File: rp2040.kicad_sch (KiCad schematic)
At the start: 8 parts, among them U1 RP2040, Y1 12 MHz

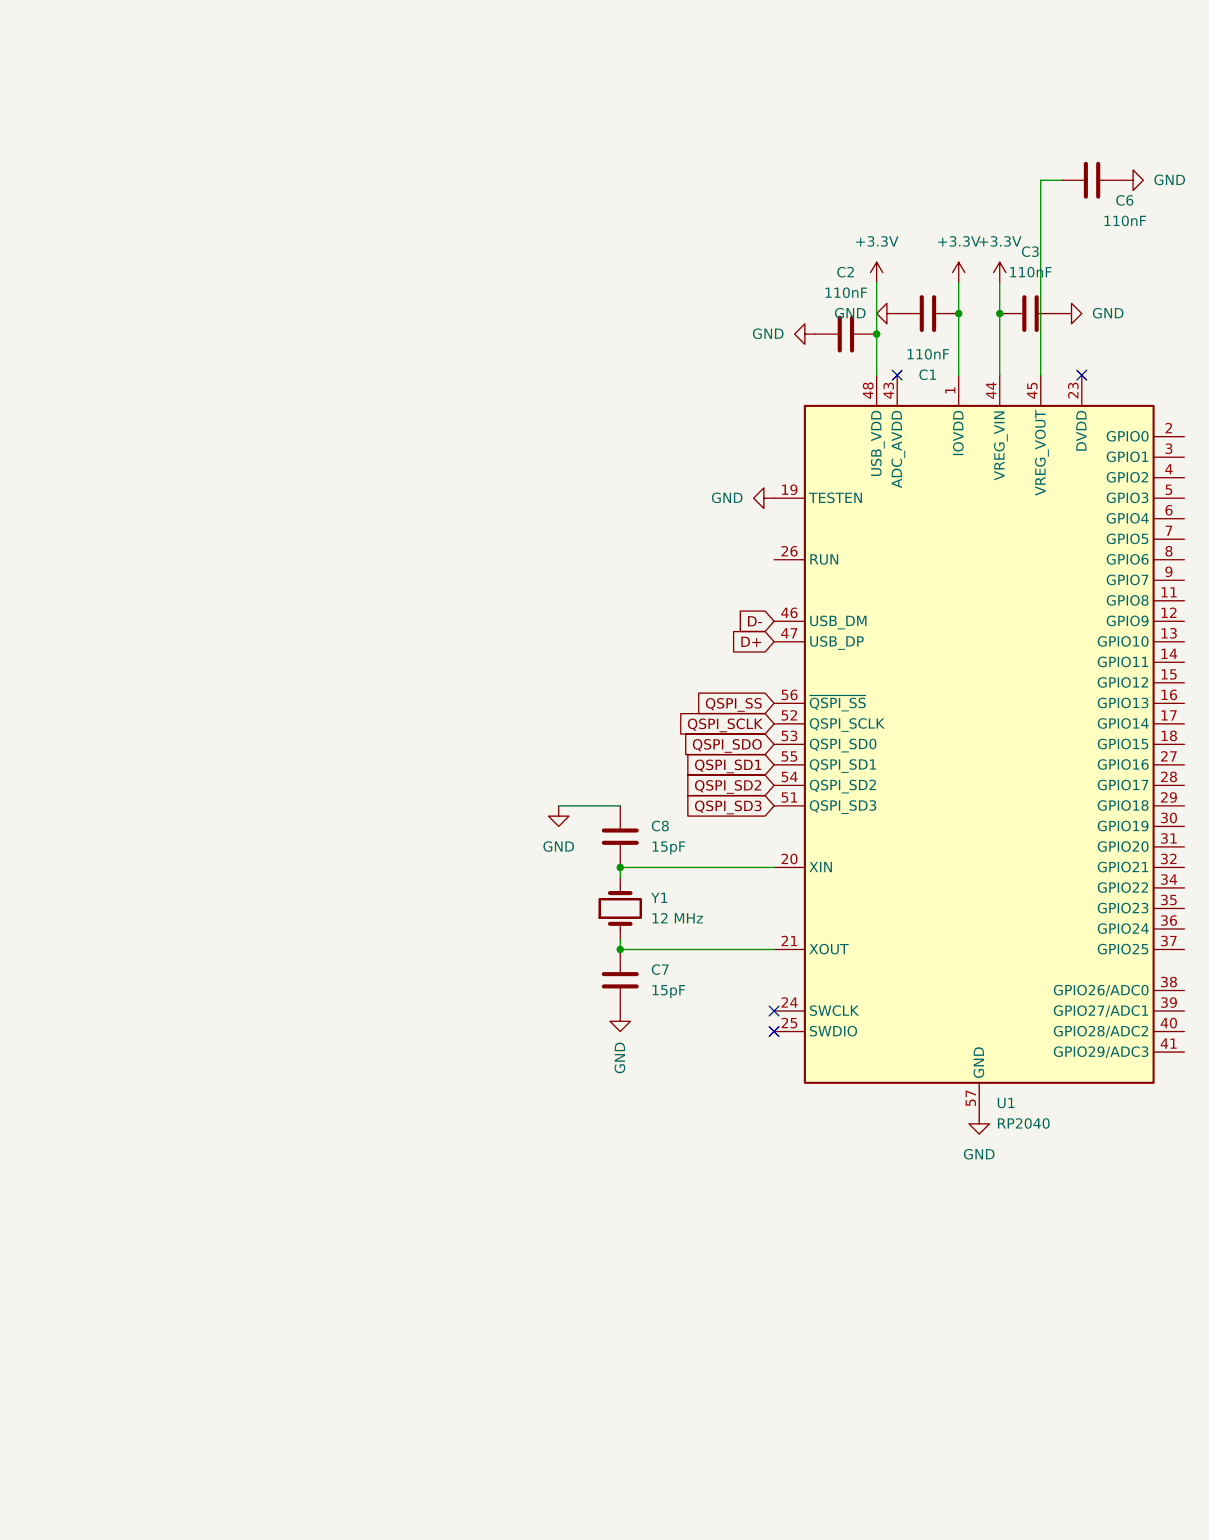
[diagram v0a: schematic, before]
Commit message: Savepoint!
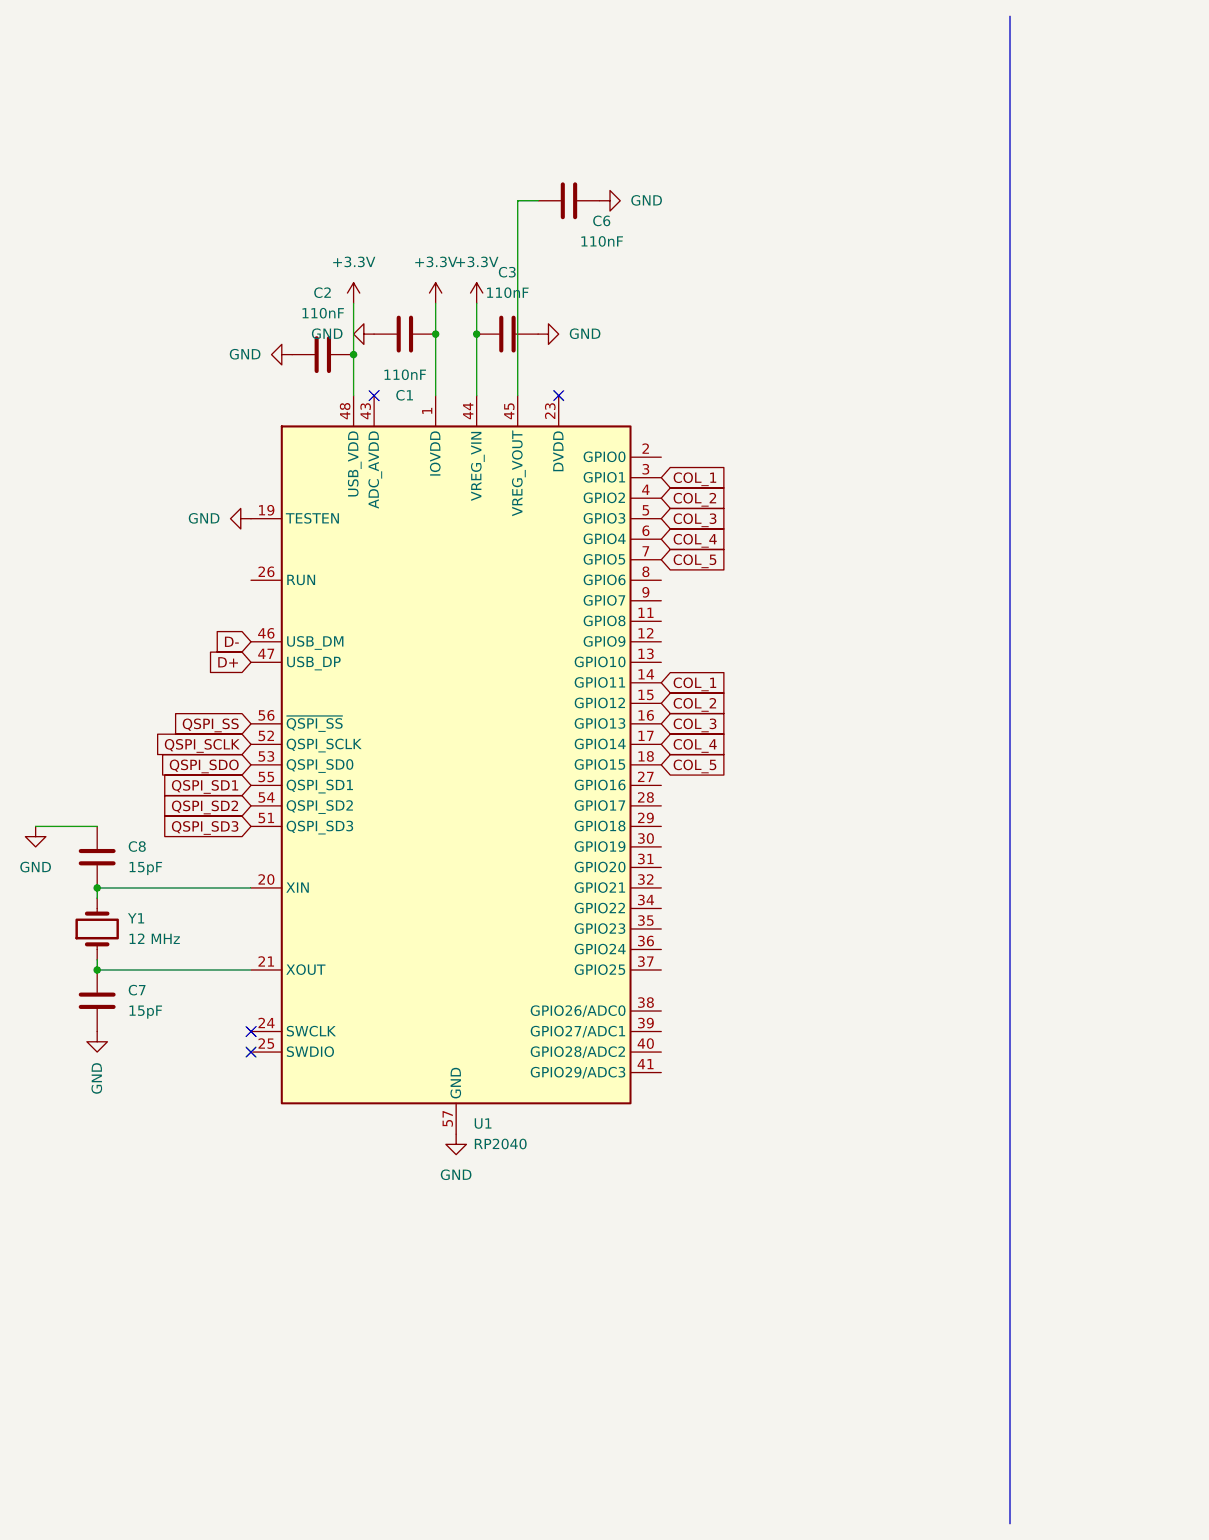
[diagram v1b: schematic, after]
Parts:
- C1, C2, C3, C6: footprint (none) -> Capacitor_Tantalum_SMD:CP_EIA-1608-08_AVX-J_HandSolder
- C7, C8: footprint (none) -> Capacitor_SMD:C_0402_1005Metric_Pad0.74x0.62mm_HandSolder
- Y1: footprint (none) -> Crystal:Crystal_SMD_3225-4Pin_3.2x2.5mm_HandSoldering
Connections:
- net COL_1: now reaches U1.14 (GPIO11)
- net COL_1: now also U1.3 (GPIO1)
- net COL_2: now reaches U1.15 (GPIO12)
- net COL_2: now also U1.4 (GPIO2)
- net COL_3: now reaches U1.16 (GPIO13)
- net COL_3: now also U1.5 (GPIO3)
- net COL_4: now reaches U1.17 (GPIO14)
- net COL_4: now also U1.6 (GPIO4)
- net COL_5: now reaches U1.18 (GPIO15)
- net COL_5: now also U1.7 (GPIO5)
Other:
- moved on the sheet: C1, C2, C3, C6, C7, C8, U1, Y1

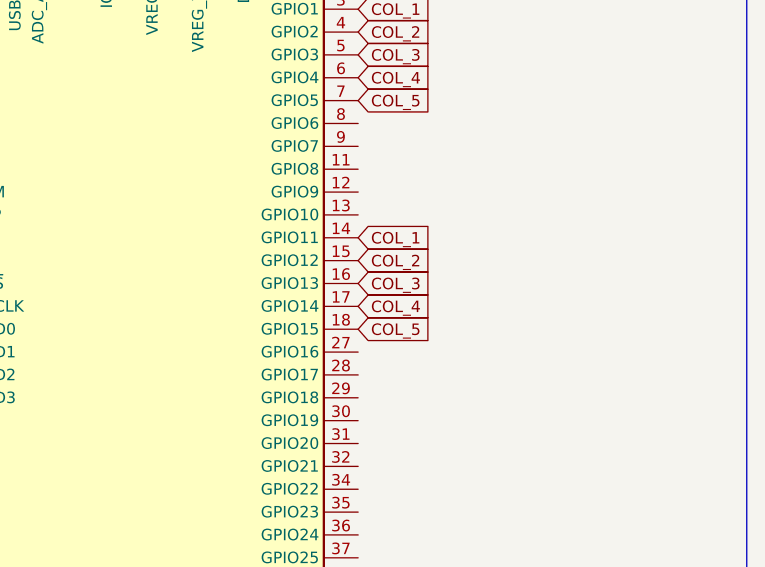
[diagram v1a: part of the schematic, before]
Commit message: Savepoint!
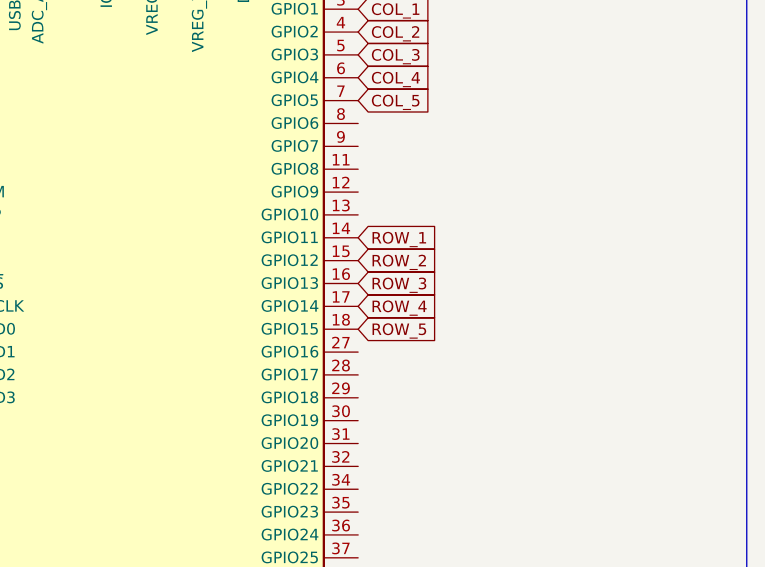
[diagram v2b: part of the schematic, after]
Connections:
- net COL_1: no longer U1.14 (GPIO11)
- net COL_2: no longer U1.15 (GPIO12)
- net COL_3: no longer U1.16 (GPIO13)
- net COL_4: no longer U1.17 (GPIO14)
- net COL_5: no longer U1.18 (GPIO15)
- new net ROW_1: U1.14 (GPIO11)
- new net ROW_2: U1.15 (GPIO12)
- new net ROW_3: U1.16 (GPIO13)
- new net ROW_4: U1.17 (GPIO14)
- new net ROW_5: U1.18 (GPIO15)
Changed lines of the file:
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@@
+		)
+	)
+	(global_label "ROW_3"
+		(shape input)
+		(at 105.41 99.06 0)
+		(fields_autoplaced yes)
+		(effects
+			(font
+				(size 1.27 1.27)
+			)
+			(justify left)
+		)
+		(property "Intersheetrefs" "${INTERSHEET_REFS}"
+			(at 114.6242 99.06 0)
+			(hide yes)
+			(show_name no)
+			(do_not_autoplace no)
+			(effects
+				(font
+					(size 1.27 1.27)
+				)
+				(justify left)
+			)
+		)
+	)
+	(global_label "QSPI_SD3"
+		(shape input)
+		(at 54.61 111.76 180)
+		(fields_autoplaced yes)
+		(effects
+			(font
+				(size 1.27 1.27)
+			)
+			(justify right)
+		)
+		(property "Intersheetrefs" "${INTERSHEET_REFS}"
+			(at 42.5534 111.76 0)
+			(hide yes)
+			(show_name no)
+			(do_not_autoplace no)
+			(effects
+				(font
+					(size 1.27 1.27)
+				)
+				(justify right)
+			)
+		)
+	)
+	(global_label "QSPI_SD2"
+		(shape input)
+		(at 54.61 109.22 180)
+		(fields_autoplaced yes)
+		(effects
+			(font
+				(size 1.27 1.27)
+			)
+			(justify right)
+		)
+		(property "Intersheetrefs" "${INTERSHEET_REFS}"
+			(at 42.5534 109.22 0)
+			(hide yes)
+			(show_name no)
+			(do_not_autoplace no)
+			(effects
+				(font
+					(size 1.27 1.27)
+				)
+				(justify right)
+			)
+		)
+	)
+	(global_label "COL_1"
+		(shape input)
+		(at 105.41 68.58 0)
+		(fields_autoplaced yes)
+		(effects
+			(font
+				(size 1.27 1.27)
+			)
+			(justify left)
+		)
+		(property "Intersheetrefs" "${INTERSHEET_REFS}"
+			(at 114.2009 68.58 0)
+			(hide yes)
+			(show_name no)
+			(do_not_autoplace no)
+			(effects
+				(font
+					(size 1.27 1.27)
+				)
+				(justify left)
+			)
+		)
+	)
+	(global_label "COL_2"
+		(shape input)
+		(at 105.41 71.12 0)
+		(fields_autoplaced yes)
+		(effects
+			(font
+				(size 1.27 1.27)
+			)
+			(justify left)
+		)
+		(property "Intersheetrefs" "${INTERSHEET_REFS}"
+			(at 114.2009 71.12 0)
+			(hide yes)
+			(show_name no)
+			(do_not_autoplace no)
+			(effects
+				(font
+					(size 1.27 1.27)
+				)
+				(justify left)
+			)
+		)
+	)
+	(global_label "ROW_5"
+		(shape input)
+		(at 105.41 104.14 0)
+		(fields_autoplaced yes)
+		(effects
+			(font
+				(size 1.27 1.27)
+			)
+			(justify left)
+		)
+		(property "Intersheetrefs" "${INTERSHEET_REFS}"
+			(at 114.6242 104.14 0)
+			(hide yes)
+			(show_name no)
+			(do_not_autoplace no)
+			(effects
+				(font
+					(size 1.27 1.27)
+				)
+				(justify left)
+			)
+		)
+	)
+	(global_label "COL_5"
+		(shape input)
+		(at 105.41 78.74 0)
+		(fields_autoplaced yes)
+		(effects
+			(font
+				(size 1.27 1.27)
+			)
+			(justify left)
+		)
+		(property "Intersheetrefs" "${INTERSHEET_REFS}"
+			(at 114.2009 78.74 0)
+			(hide yes)
+			(show_name no)
+			(do_not_autoplace no)
+			(effects
+				(font
+					(size 1.27 1.27)
+				)
+				(justify left)
+			)
+		)
+	)
+	(global_label "QSPI_SS"
+		(shape input)
+		(at 54.61 99.06 180)
+		(fields_autoplaced yes)
+		(effects
+			(font
+				(size 1.27 1.27)
+			)
+			(justify right)
+		)
+		(property "Intersheetrefs" "${INTERSHEET_REFS}"
+			(at 43.8234 99.06 0)
+			(hide yes)
+			(show_name no)
+			(do_not_autoplace no)
+			(effects
+				(font
+					(size 1.27 1.27)
+				)
+				(justify right)
+			)
 		)
 	)
 	(global_label "COL_3"
 		(shape input)
-		(at 105.41 99.06 0)
-		(fields_autoplaced yes)
-		(effects
-			(font
-				(size 1.27 1.27)
-			)
-			(justify left)
-		)
-		(property "Intersheetrefs" "${INTERSHEET_REFS}"
-			(at 114.2009 99.06 0)
-			(hide yes)
-			(show_name no)
-			(do_not_autoplace no)
-			(effects
-				(font
-					(size 1.27 1.27)
-				)
-				(justify left)
-			)
-		)
-	)
-	(global_label "QSPI_SD3"
-		(shape input)
-		(at 54.61 111.76 180)
-		(fields_autoplaced yes)
-		(effects
-			(font
-				(size 1.27 1.27)
-			)
-			(justify right)
-		)
-		(property "Intersheetrefs" "${INTERSHEET_REFS}"
-			(at 42.5534 111.76 0)
-			(hide yes)
-			(show_name no)
-			(do_not_autoplace no)
-			(effects
-				(font
-					(size 1.27 1.27)
-				)
-				(justify right)
-			)
-		)
-	)
-	(global_label "QSPI_SD2"
-		(shape input)
-		(at 54.61 109.22 180)
-		(fields_autoplaced yes)
-		(effects
-			(font
-				(size 1.27 1.27)
-			)
-			(justify right)
-		)
-		(property "Intersheetrefs" "${INTERSHEET_REFS}"
-			(at 42.5534 109.22 0)
-			(hide yes)
-			(show_name no)
-			(do_not_autoplace no)
-			(effects
-				(font
-					(size 1.27 1.27)
-				)
-				(justify right)
-			)
-		)
-	)
-	(global_label "COL_1"
-		(shape input)
-		(at 105.41 68.58 0)
-		(fields_autoplaced yes)
-		(effects
-			(font
-				(size 1.27 1.27)
-			)
-			(justify left)
-		)
-		(property "Intersheetrefs" "${INTERSHEET_REFS}"
-			(at 114.2009 68.58 0)
-			(hide yes)
-			(show_name no)
-			(do_not_autoplace no)
-			(effects
-				(font
-					(size 1.27 1.27)
-				)
-				(justify left)
-			)
-		)
-	)
-	(global_label "COL_2"
-		(shape input)
-		(at 105.41 71.12 0)
-		(fields_autoplaced yes)
-		(effects
-			(font
-				(size 1.27 1.27)
-			)
-			(justify left)
-		)
-		(property "Intersheetrefs" "${INTERSHEET_REFS}"
-			(at 114.2009 71.12 0)
-			(hide yes)
-			(show_name no)
-			(do_not_autoplace no)
-			(effects
-				(font
-					(size 1.27 1.27)
-				)
-				(justify left)
-			)
-		)
-	)
-	(global_label "COL_5"
-		(shape input)
-		(at 105.41 104.14 0)
-		(fields_autoplaced yes)
-		(effects
-			(font
-				(size 1.27 1.27)
-			)
-			(justify left)
-		)
-		(property "Intersheetrefs" "${INTERSHEET_REFS}"
-			(at 114.2009 104.14 0)
-			(hide yes)
-			(show_name no)
-			(do_not_autoplace no)
-			(effects
-				(font
-					(size 1.27 1.27)
-				)
-				(justify left)
-			)
-		)
-	)
-	(global_label "COL_5"
-		(shape input)
-		(at 105.41 78.74 0)
-		(fields_autoplaced yes)
-		(effects
-			(font
-				(size 1.27 1.27)
-			)
-			(justify left)
-		)
-		(property "Intersheetrefs" "${INTERSHEET_REFS}"
-			(at 114.2009 78.74 0)
-			(hide yes)
-			(show_name no)
-			(do_not_autoplace no)
-			(effects
-				(font
-					(size 1.27 1.27)
-				)
-				(justify left)
-			)
-		)
-	)
-	(global_label "QSPI_SS"
-		(shape input)
-		(at 54.61 99.06 180)
-		(fields_autoplaced yes)
-		(effects
-			(font
-				(size 1.27 1.27)
-			)
-			(justify right)
-		)
-		(property "Intersheetrefs" "${INTERSHEET_REFS}"
-			(at 43.8234 99.06 0)
-			(hide yes)
-			(show_name no)
-			(do_not_autoplace no)
-			(effects
-				(font
-					(size 1.27 1.27)
-				)
-				(justify right)
-			)
-		)
-	)
-	(global_label "COL_3"
-		(shape input)
 		(at 105.41 73.66 0)
 		(fields_autoplaced yes)
@@
 		)
 	)
-	(global_label "COL_4"
+	(global_label "ROW_4"
 		(shape input)
 		(at 105.41 101.6 0)
@@
 		)
 		(property "Intersheetrefs" "${INTERSHEET_REFS}"
-			(at 114.2009 101.6 0)
-			(hide yes)
-			(show_name no)
-			(do_not_autoplace no)
-			(effects
-				(font
-					(size 1.27 1.27)
-				)
-				(justify left)
-			)
-		)
-	)
-	(global_label "COL_2"
+			(at 114.6242 101.6 0)
+			(hide yes)
+			(show_name no)
+			(do_not_autoplace no)
+			(effects
+				(font
+					(size 1.27 1.27)
+				)
+				(justify left)
+			)
+		)
+	)
+	(global_label "ROW_2"
 		(shape input)
 		(at 105.41 96.52 0)
@@
 		)
 		(property "Intersheetrefs" "${INTERSHEET_REFS}"
-			(at 114.2009 96.52 0)
+			(at 114.6242 96.52 0)
 			(hide yes)
 			(show_name no)
@@
 		)
 	)
-	(global_label "COL_1"
+	(global_label "ROW_1"
 		(shape input)
 		(at 105.41 93.98 0)
@@
 		)
 		(property "Intersheetrefs" "${INTERSHEET_REFS}"
-			(at 114.2009 93.98 0)
-			(hide yes)
-			(show_name no)
+			(at 114.6242 93.98 0)
+			(hide yes)
+			(show_name no)

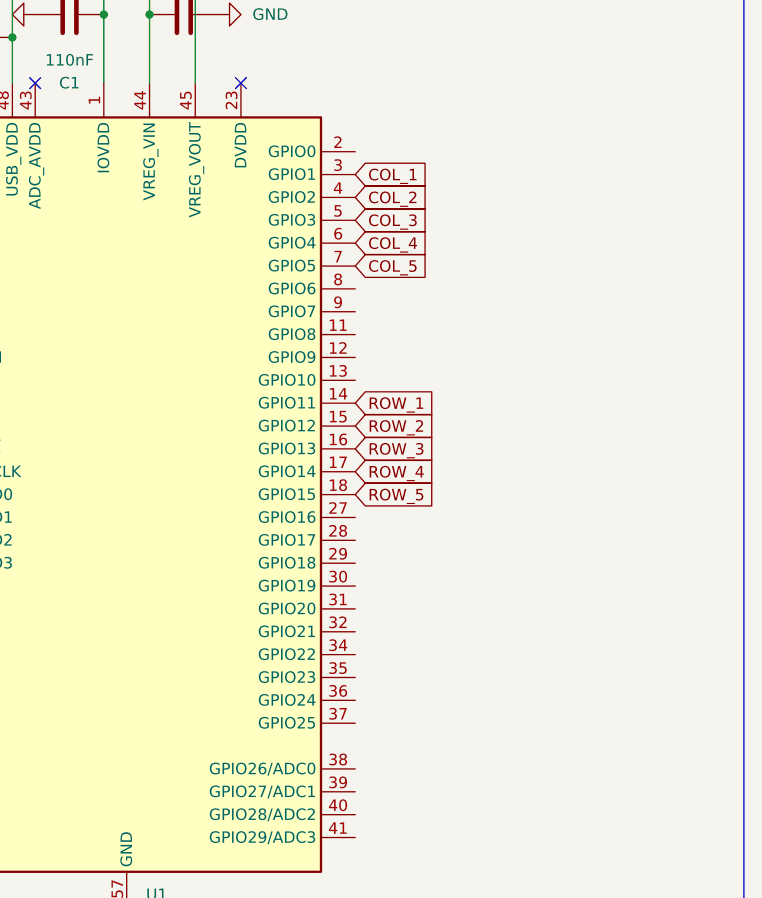
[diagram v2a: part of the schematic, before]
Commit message: Savepoint!
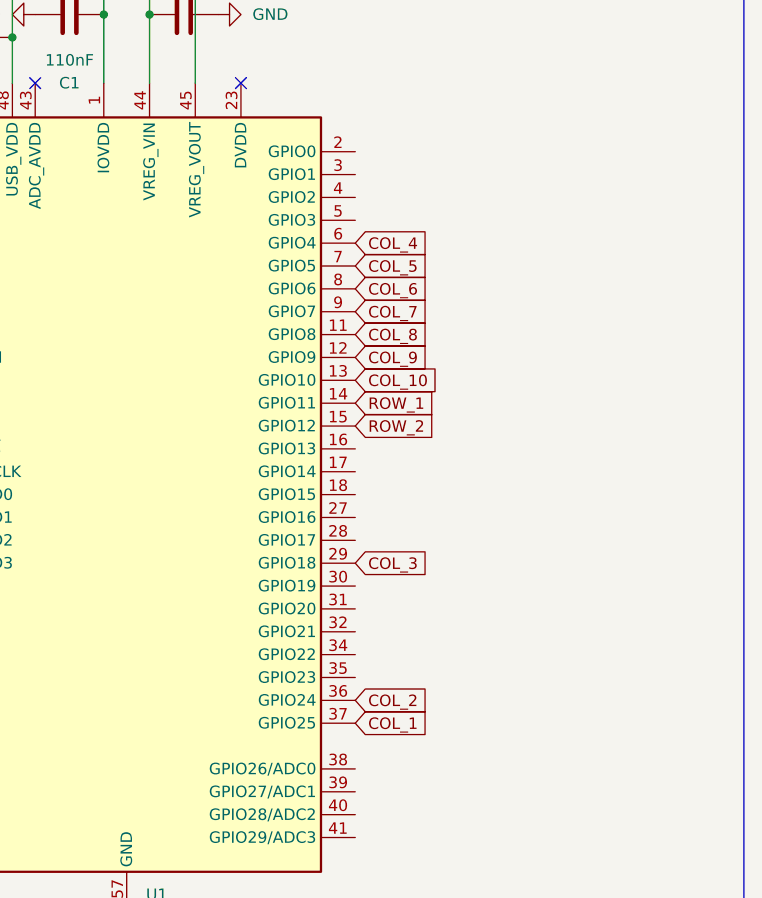
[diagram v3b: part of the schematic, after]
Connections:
- net COL_1: now also U1.37 (GPIO25); no longer U1.3 (GPIO1)
- net COL_2: now also U1.36 (GPIO24); no longer U1.4 (GPIO2)
- net COL_3: now also U1.29 (GPIO18); no longer U1.5 (GPIO3)
- net COL_8: now reaches U1.11 (GPIO8)
- net COL_9: now reaches U1.12 (GPIO9)
- net COL_10: now reaches U1.13 (GPIO10)
- net COL_6: now reaches U1.8 (GPIO6)
- net COL_7: now reaches U1.9 (GPIO7)
- net ROW_3: no longer names the net of U1.16 (GPIO13)
- net ROW_4: no longer names the net of U1.17 (GPIO14)
- net ROW_5: no longer names the net of U1.18 (GPIO15)
